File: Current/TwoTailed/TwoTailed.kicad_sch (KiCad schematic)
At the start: 38 parts, among them J1 USB, J2 I2C, U0 RP2040, U1 LDO-3.3, U2 USBLC6-2SC6, U3 W25Q128JVS, Y1 12MHz

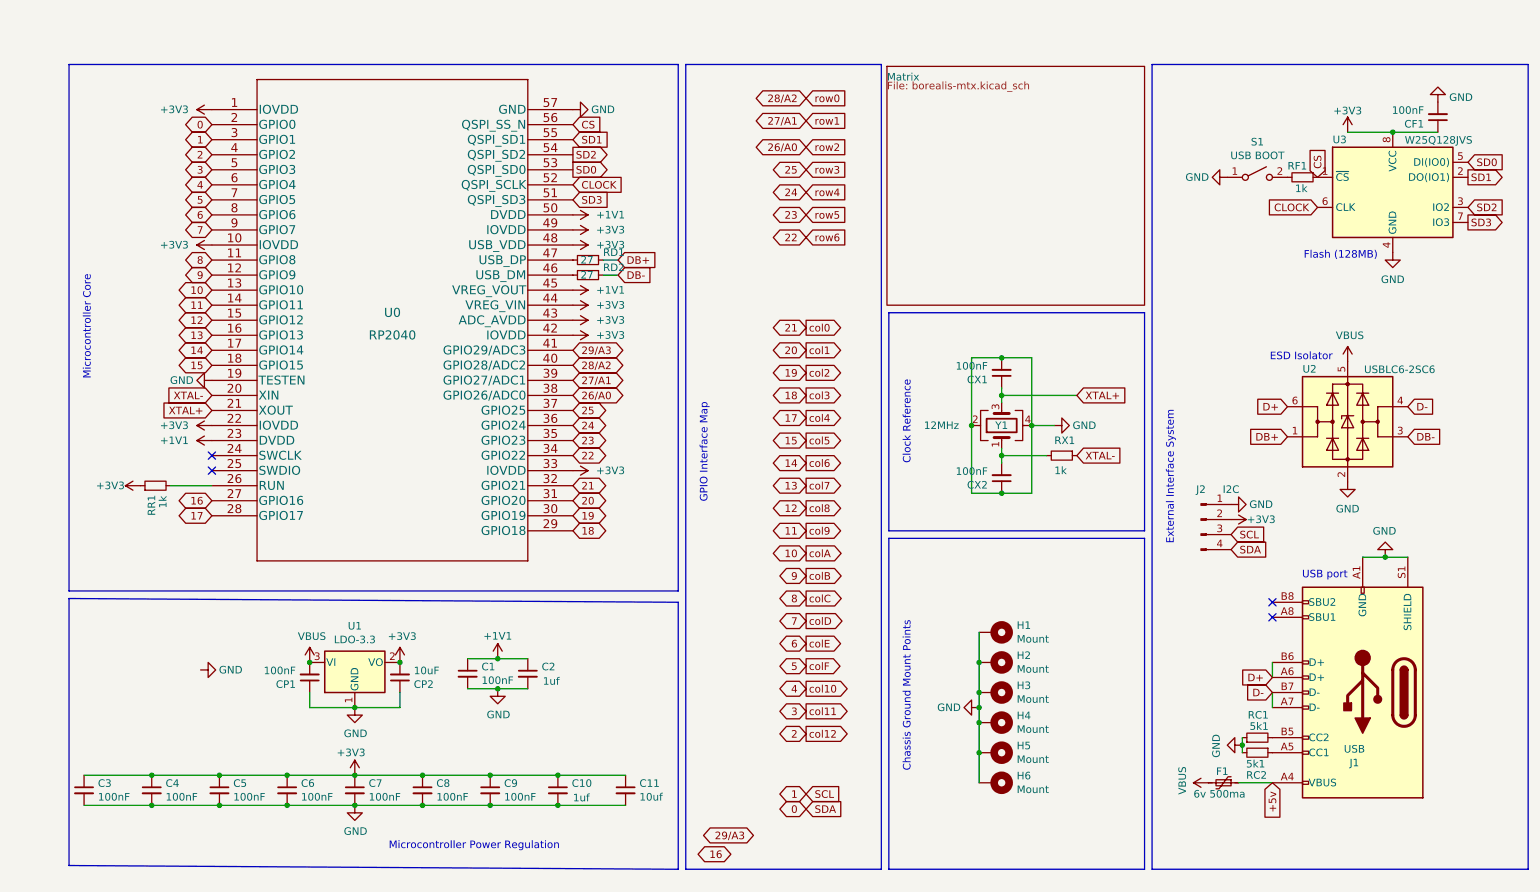
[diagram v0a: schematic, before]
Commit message: So much stuff
Wow it's been a while.
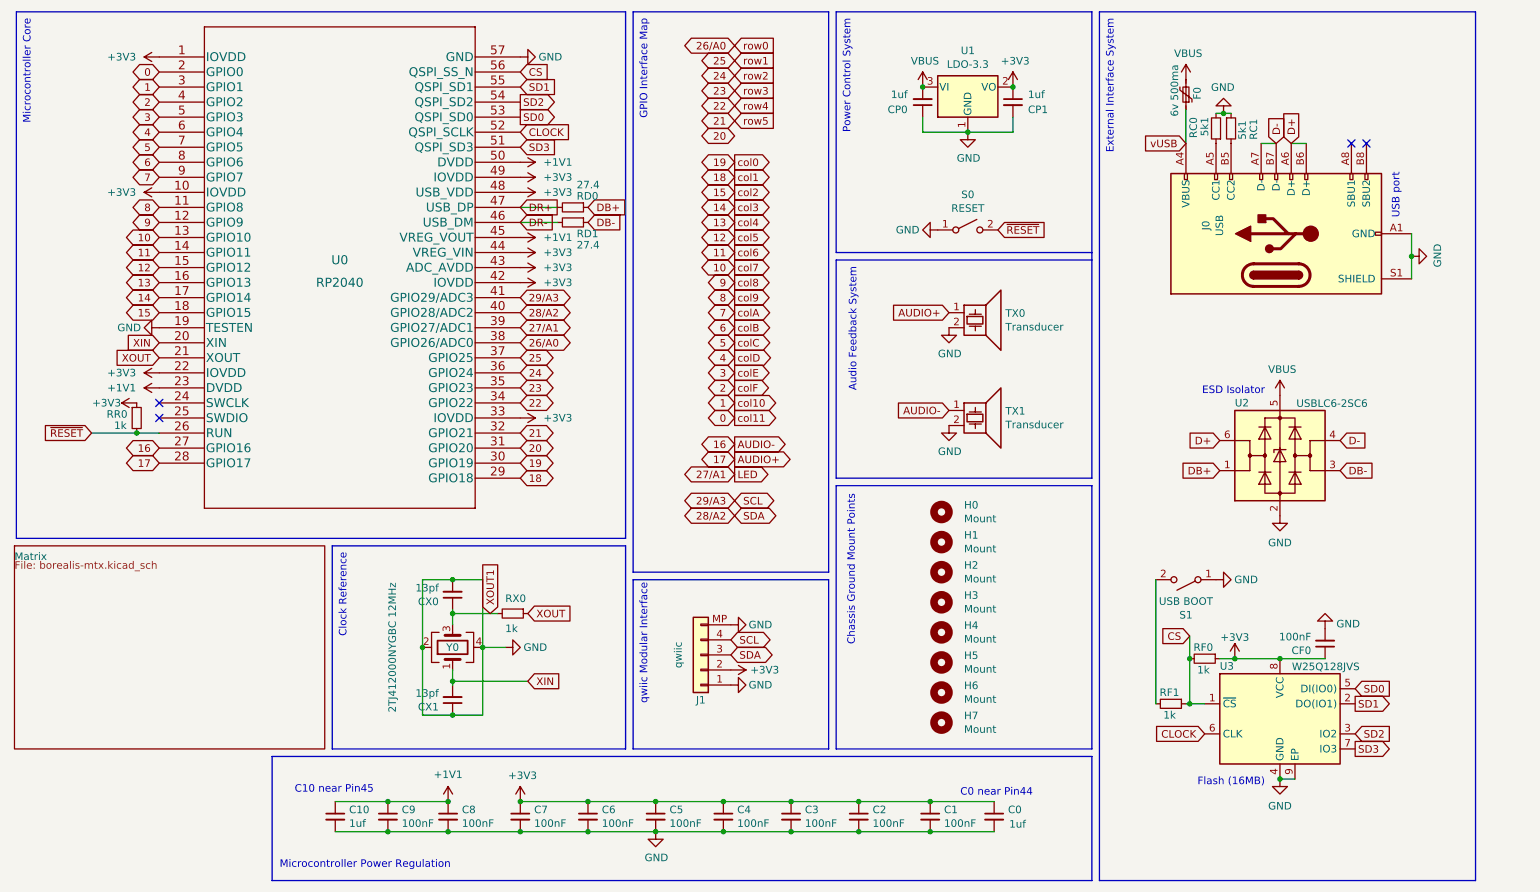
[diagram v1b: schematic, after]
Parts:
- removed C11: 10uf, EDI:Passive_0402_1005Metric, symbol Device:C_Small
- removed CF1, CX2: 100nF, EDI:Passive_0402_1005Metric, symbol Device:C_Small
- removed CP2: 10uF, EDI:Passive_0402_1005Metric, symbol Device:C_Small
- removed F1: 6v 500ma, Fuse:Fuse_0603_1608Metric, symbol Device:Polyfuse_Small
- removed H1, H2, H3, H4, H5, H6: Mount, EDI:SolderableHole, symbol Mechanical:MountingHole_Pad
- removed J1: USB, Connector_USB:USB_C_Receptacle_HRO_TYPE-C-31-M-12, symbol HL-Mk2-rescue:USB_C_Receptacle_USB2.0-Connector
- removed J2: I2C, Connector_PinHeader_2.54mm:PinHeader_1x04_P2.54mm_Vertical, symbol Connector:Conn_01x04_Male
- removed RC2: 5k1, EDI:Passive_0402_1005Metric, symbol Device:R_Small
- removed RD2: 27, EDI:Passive_0402_1005Metric, symbol Device:R_Small
- removed RR1, RX1: 1k, EDI:Passive_0402_1005Metric, symbol Device:R_Small
- removed U3: W25Q128JVS, Package_SO:SOIC-8_5.23x5.23mm_P1.27mm, symbol Memory_Flash:W25Q128JVS
- removed Y1: 12MHz, Crystal:Crystal_SMD_3225-4Pin_3.2x2.5mm, symbol Device:Crystal_GND24
- added C0, CP0: 1uf, EDI:Passive_0402_1005Metric, symbol Device:C_Small
- added CF0: 100nF, EDI:Passive_0402_1005Metric, symbol Device:C_Small
- added CX0: 13pf, EDI:Passive_0402_1005Metric, symbol Device:C_Small
- added F0: 6v 500ma, Fuse:Fuse_0603_1608Metric, symbol Device:Polyfuse_Small
- added H0, H1, H2, H3, H4, H5, H6, H7: Mount, MountingHole:MountingHole_3.2mm_M3, symbol Mechanical:MountingHole
- added J0: USB, Connector_USB:USB_C_Receptacle_HRO_TYPE-C-31-M-12, symbol HL-Mk2-rescue:USB_C_Receptacle_USB2.0-Connector
- added J1: qwiic, Connector_JST:JST_SH_SM04B-SRSS-TB_1x04-1MP_P1.00mm_Horizontal, symbol Connector_Generic:Conn_01x05
- added RC0: 5k1, EDI:Passive_0402_1005Metric, symbol Device:R_Small
- added RD0: 27.4, EDI:Passive_0402_1005Metric, symbol Device:R_Small
- added RF0, RR0, RX0: 1k, EDI:Passive_0402_1005Metric, symbol Device:R_Small
- added S0: RESET, Button_Switch_SMD:SW_SPST_SKQG_WithoutStem, symbol Switch:SW_SPST
- added TX0, TX1: Transducer, Buzzer_Beeper:Buzzer_CUI_CPT-9019S-SMT, symbol Device:Speaker_Crystal
- added U3: W25Q128JVS, Package_SON:WSON-8-1EP_6x5mm_P1.27mm_EP3.4x4.3mm, symbol Memory_Flash:W25Q32JVZP
- added Y0: 2TJ412000NYGBC 12MHz, Crystal:Crystal_SMD_2520-4Pin_2.5x2.0mm, symbol Device:Crystal_GND24
- C2: value 1uf -> 100nF; LCSC C52923 -> C1525
- CP1: value 100nF -> 1uf; LCSC C1525 -> C52923
- CX1: value 100nF -> 13pf; LCSC C1525 -> C48936
- RD1: value 27 -> 27.4; LCSC C413051 -> C172043
- S1: footprint EDI:SW_EVPBB4A9B000 -> Button_Switch_SMD:SW_SPST_SKQG_WithoutStem; LCSC C140848 -> C139779
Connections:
- net +1V1: now also C10.1, C8.1, C9.1; no longer C1.1, C2.1
- net +3V3: now also C1.1, C2.1, CP1.1, C0.1, CF0.1, J1.2 (Pin_2), RF0.1, RR0.1, U3.8 (VCC); no longer C10.1, C8.1, C9.1
- net 16: now also TX1.1
- net 17: now also TX0.1
- net 28/A2: now also J1.3 (Pin_3)
- net 29/A3: now also J1.4 (Pin_4)
- net CLOCK: now also U3.6 (CLK)
- net CS: now also RF0.2, U3.1 (~{CS})
- net D+: now also J0.A6 (D+), J0.B6 (D+)
- net D-: now also J0.A7 (D-), J0.B7 (D-)
- net DB+: now also RD0.1; no longer RD1.1
- net DB-: now also RD1.1
- net GND: now also CP1.2, CX1.1, C0.2, CF0.2, CP0.1, CX0.2, J0.A1 (GND), J0.A12 (GND), J0.B1 (GND), J0.B12 (GND), J0.S1 (SHIELD), J1.1 (Pin_1), J1.MP, RC0.2, S0.1 (A), TX0.2, TX1.2, U3.4 (GND), U3.9 (EP), Y0.2, Y0.4; no longer CP1.1, CX1.2
- net SD0: now also U3.5 (DI(IO0))
- net SD1: now also U3.2 (DO(IO1))
- net SD2: now also U3.3 (IO2)
- net SD3: now also U3.7 (IO3)
- net VBUS: now also CP0.2, F0.2; no longer CP1.2
- net DR+: now reaches U0.47 (USB_DP)
- net DR+: now also RD0.2; no longer RD1.2
- net DR-: now reaches U0.46 (USB_DM)
- net DR-: now also RD1.2
- net ~{RESET}: now reaches U0.26 (RUN)
- net ~{RESET}: now also RR0.2, S0.2 (B)
- net at RC1.2: now also J0.B5 (CC2)
- net XTAL+ renamed XOUT
- net XOUT: now also RX0.1; no longer CX1.1
- net XTAL- renamed XIN
- net XIN: now also CX1.2, Y0.1
- new net: J0.A5 (CC1), RC0.1
- new net XOUT1: CX0.1, RX0.2, Y0.3
- new net vUSB: F0.1, J0.A4 (VBUS), J0.A9 (VBUS), J0.B4 (VBUS), J0.B9 (VBUS)
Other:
- note added: "Audio Feedback System"
- note added: "C0 near Pin44"
- note added: "C10 near Pin45"
- note added: "Flash (16MB)"
- note added: "Power Control System"
- note added: "qwiic Modular Interface"
- note removed: "Flash (128MB)"
